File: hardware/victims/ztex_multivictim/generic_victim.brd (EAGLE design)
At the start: 123.2 x 84.8 mm, 81 parts, among them CON1 CHIPCARD-SOCKET, IC1 ATMEGA48/88/168-PU, IC3 XMEGA16A4-AU, Q2 OSC-OSCILLATOR, Q3 OSC-OSCILLATOR, U1 BGA2801, U2 BGA2801, X1 BU-SMA-V, X2 BU-SMA-V, X3 BU-SMA-V, X4 BU-SMA-V

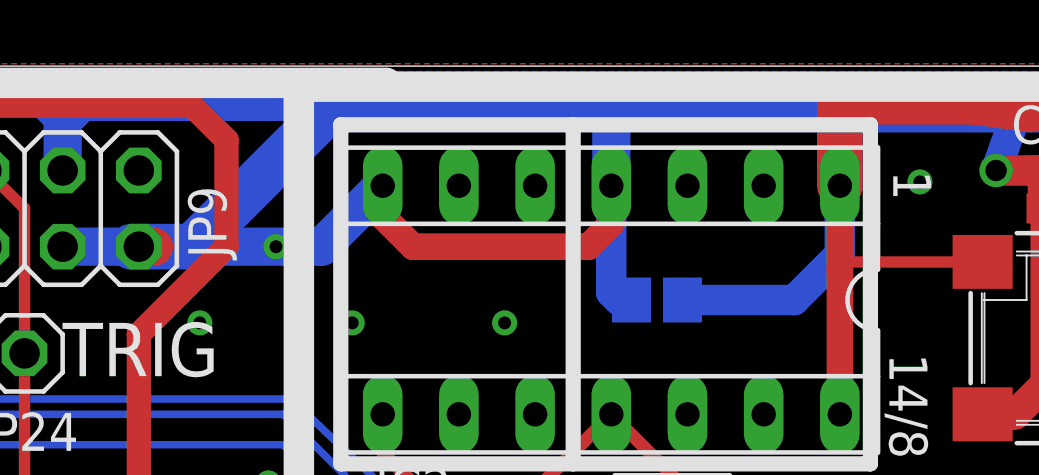
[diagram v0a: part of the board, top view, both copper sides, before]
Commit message: Fix ZTEX generic victim
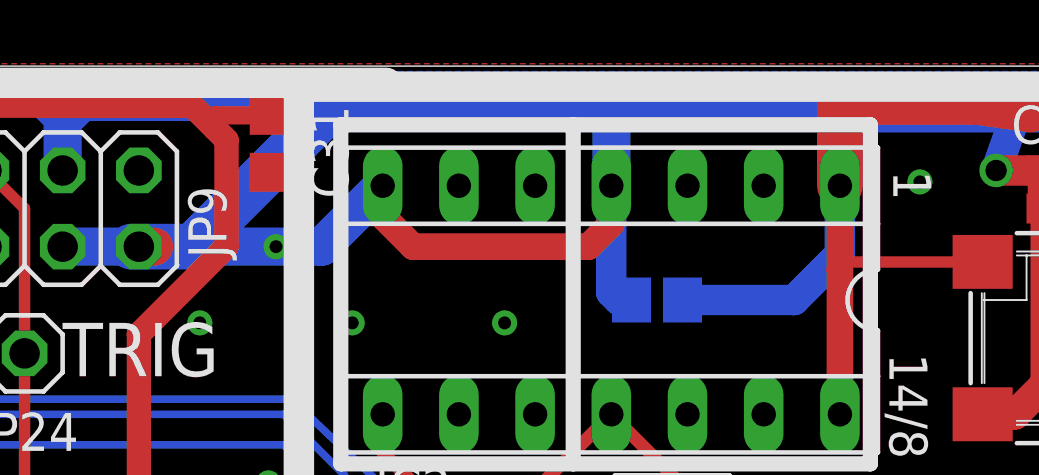
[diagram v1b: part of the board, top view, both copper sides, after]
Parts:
- added C31: 100nF, rcl:C0805
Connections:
- net GND: now also C31.2
- net VREF: now also C31.1
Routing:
- net VREF: track 69.3 -> 71.6 mm
- net +3V3: track 322.9 -> 325.0 mm
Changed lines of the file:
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@@
 <attribute name="VALUE" x="13.081" y="55.626" size="1.27" layer="27"/>
 </element>
+<element name="C31" library="rcl" package="C0805" value="100nF" x="83.693" y="87.249" rot="R270"/>
 </elements>
 <signals>
@@
 <via x="120.396" y="60.706" extent="1-16" drill="0.4318"/>
 <via x="120.396" y="64.008" extent="1-16" drill="0.4318"/>
+<contactref element="C31" pad="2"/>
 </signal>
 <signal name="N$1">
@@
 <wire x1="102.362" y1="88.646" x2="102.616" y2="88.392" width="1.27" layer="16"/>
 <wire x1="102.616" y1="88.392" x2="102.616" y2="87.884" width="1.27" layer="16"/>
-<wire x1="102.616" y1="88.392" x2="102.616" y2="88.646" width="0" layer="19" extent="1-16"/>
+<wire x1="102.616" y1="87.884" x2="102.616" y2="85.852" width="1.27" layer="16"/>
 </signal>
 <signal name="N$24">
@@
 <wire x1="64.008" y1="87.503" x2="65.024" y2="88.519" width="0.8128" layer="1"/>
 <wire x1="65.024" y1="88.519" x2="81.026" y2="88.519" width="0.8128" layer="1"/>
-<wire x1="81.026" y1="88.519" x2="82.169" y2="87.376" width="0.8128" layer="1"/>
+<wire x1="81.026" y1="88.519" x2="81.788" y2="87.757" width="0.8128" layer="1"/>
+<wire x1="81.788" y1="87.757" x2="82.169" y2="87.376" width="0.8128" layer="1"/>
 <wire x1="82.169" y1="87.376" x2="82.169" y2="83.82" width="0.8128" layer="1"/>
 <wire x1="82.169" y1="83.82" x2="79.248" y2="80.899" width="0.8128" layer="1"/>
@@
 <wire x1="81.026" y1="70.866" x2="81.026" y2="63.5" width="0.8128" layer="16"/>
 <wire x1="81.026" y1="63.5" x2="79.502" y2="61.976" width="0.8128" layer="16"/>
+<contactref element="C31" pad="1"/>
+<wire x1="83.693" y1="88.199" x2="81.788" y2="88.199" width="0.6096" layer="1"/>
+<wire x1="81.788" y1="88.199" x2="81.788" y2="87.757" width="0.6096" layer="1"/>
 </signal>
 </signals>
